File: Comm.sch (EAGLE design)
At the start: 33 parts, among them SW5 THAU13-AB-R, SW6 THAU13-AB-R, SW7 TVAF06-A020B-R, SW8 TVAF06-A020B-R, U4 OPA340N, U5 DRIVER-LV8548MC-AH(SOIC10), U6 I-02247_NJM2845

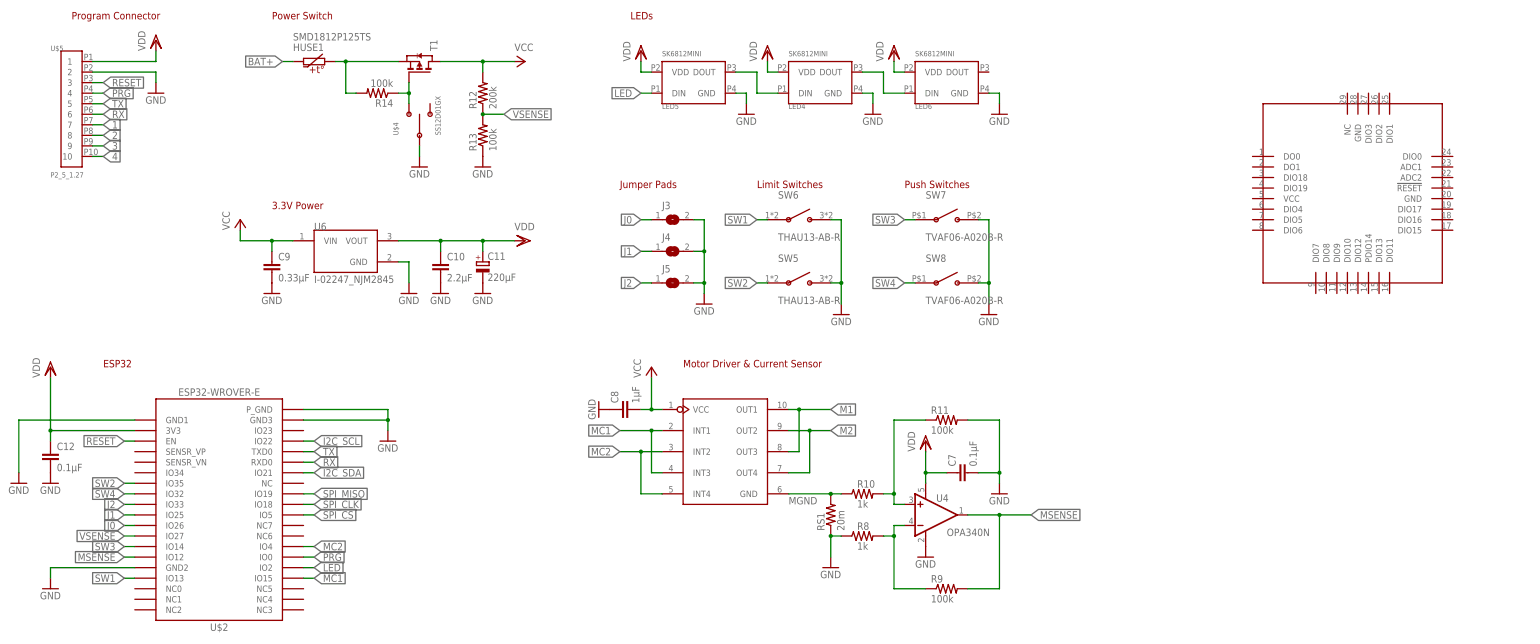
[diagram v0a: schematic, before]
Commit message: Communication unit
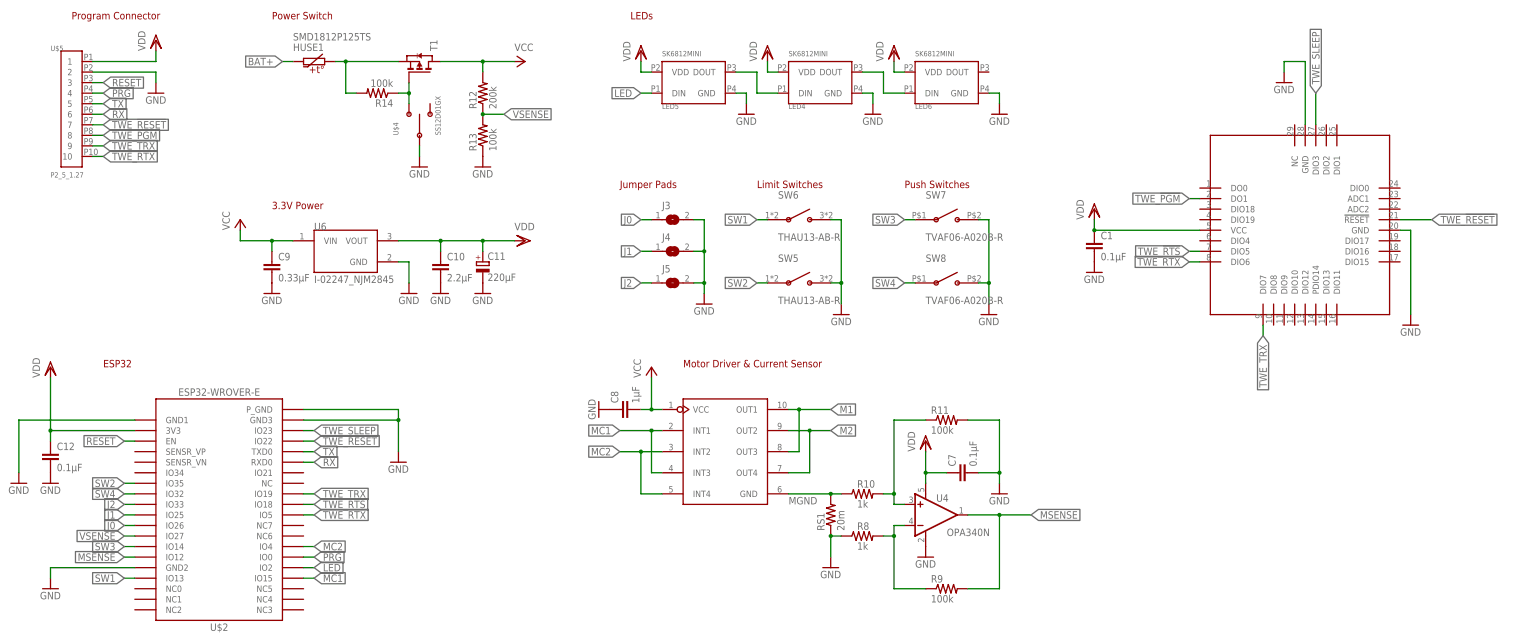
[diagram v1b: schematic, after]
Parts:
- removed U$1: LITE, TWELite:LITE
- added C1: 0.1µF, rcl:C-EUC0603K
- added TWE-LITE: LITE, TWELite:LITE
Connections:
- removed net 1: U$5.7
- removed net 2: U$5.8
- removed net 3: U$5.9
- removed net 4: U$5.10
- removed net I2C_SCL: U$2.IO22
- removed net I2C_SDA: U$2.IO21
- removed net SPI_CLK: U$2.IO18
- removed net SPI_CS: U$2.IO5
- removed net SPI_MISO: U$2.IO19
- new net TWE_!PGM!: TWE-LITE.DO1, U$5.8
- new net TWE_!RESET!: TWE-LITE.!RESET!, U$2.IO22, U$5.7
- new net TWE_!RTS!: TWE-LITE.DIO5, U$2.IO18
- new net TWE_RTX: TWE-LITE.DIO6, U$2.IO5, U$5.10
- new net TWE_SLEEP: TWE-LITE.DIO3, U$2.IO23
- new net TWE_TRX: TWE-LITE.DIO7, U$2.IO19, U$5.9
- net GND: now also C1.2, TWE-LITE.GND@1, TWE-LITE.GND@2
- net VDD: now also C1.1, TWE-LITE.VCC
